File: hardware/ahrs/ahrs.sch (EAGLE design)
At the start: 32 parts, among them J1 2-PIN, U1 LSM9DS1, U2 STM32G4_UFQFPN48_T1, X1 NX2016SA24MHZ-EXS00A-CS11335, X2 SM08B-SRSS-TB

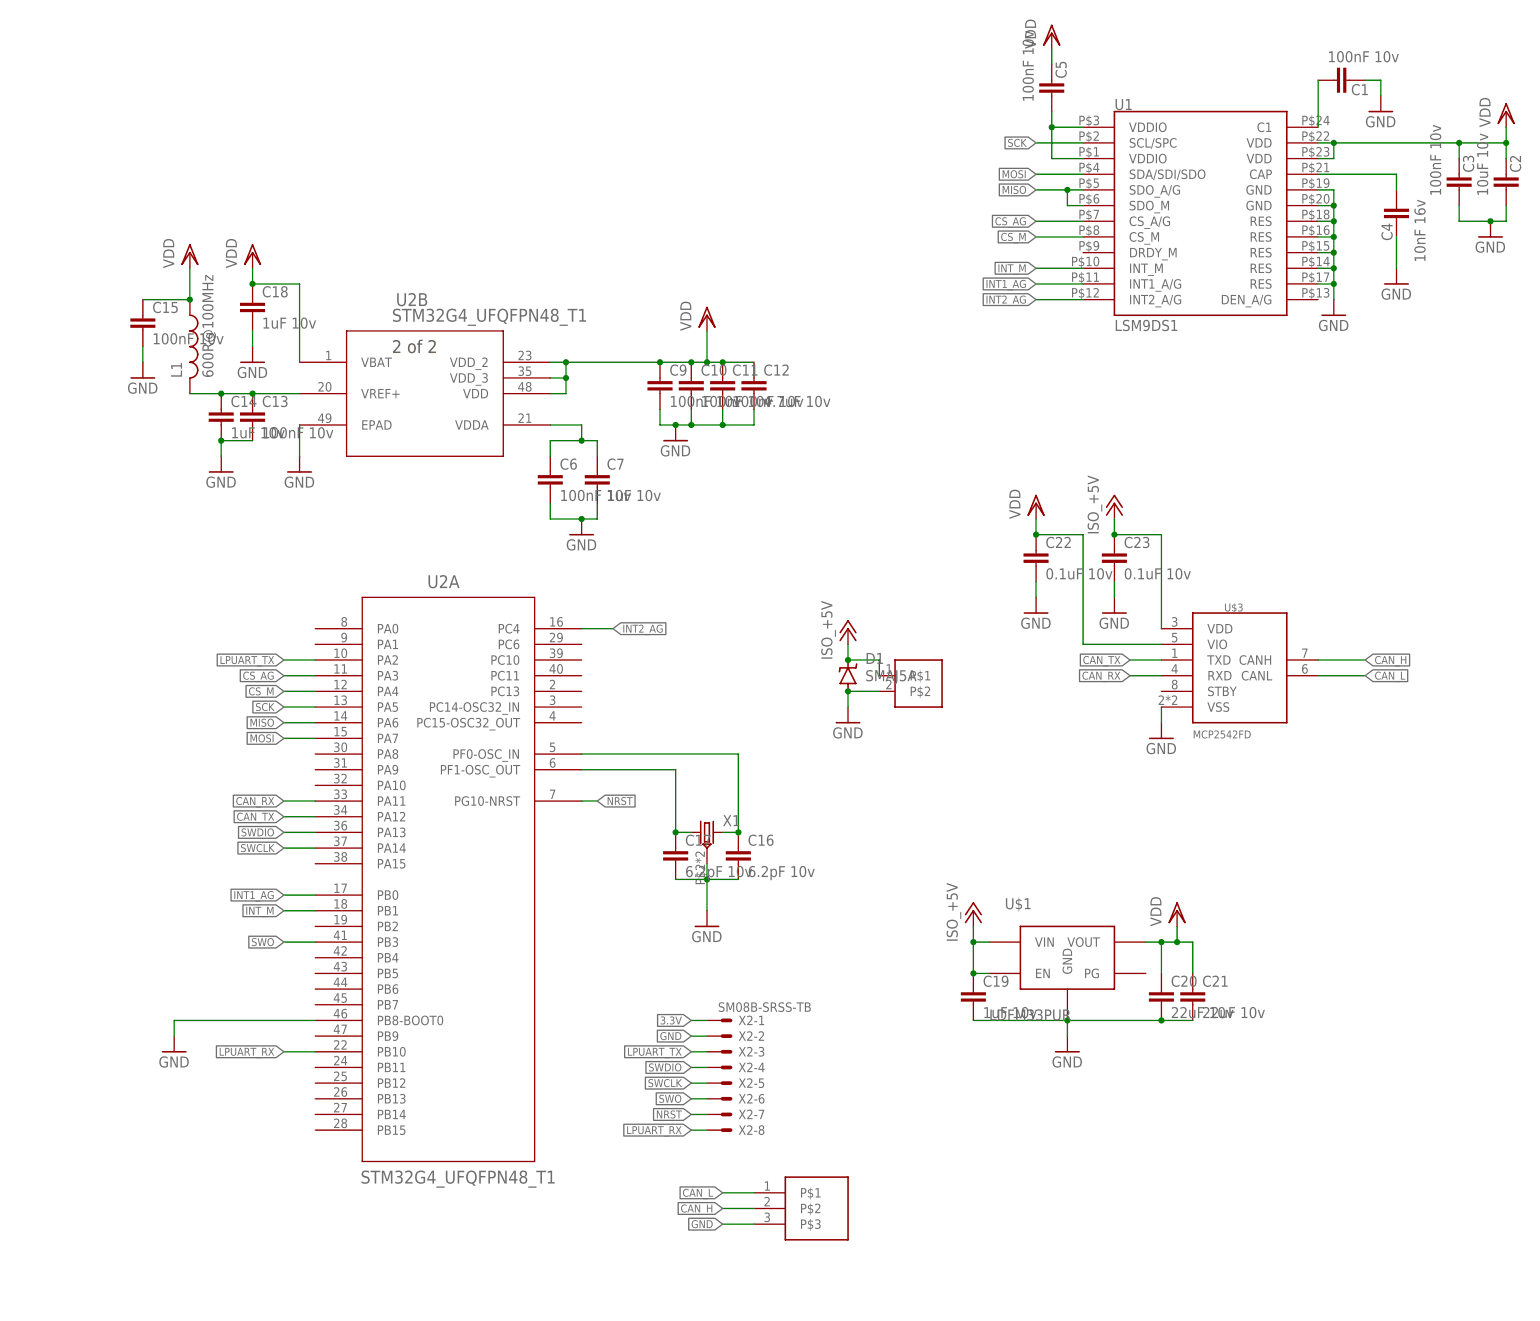
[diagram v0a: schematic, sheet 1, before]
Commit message: R1 of ahrs
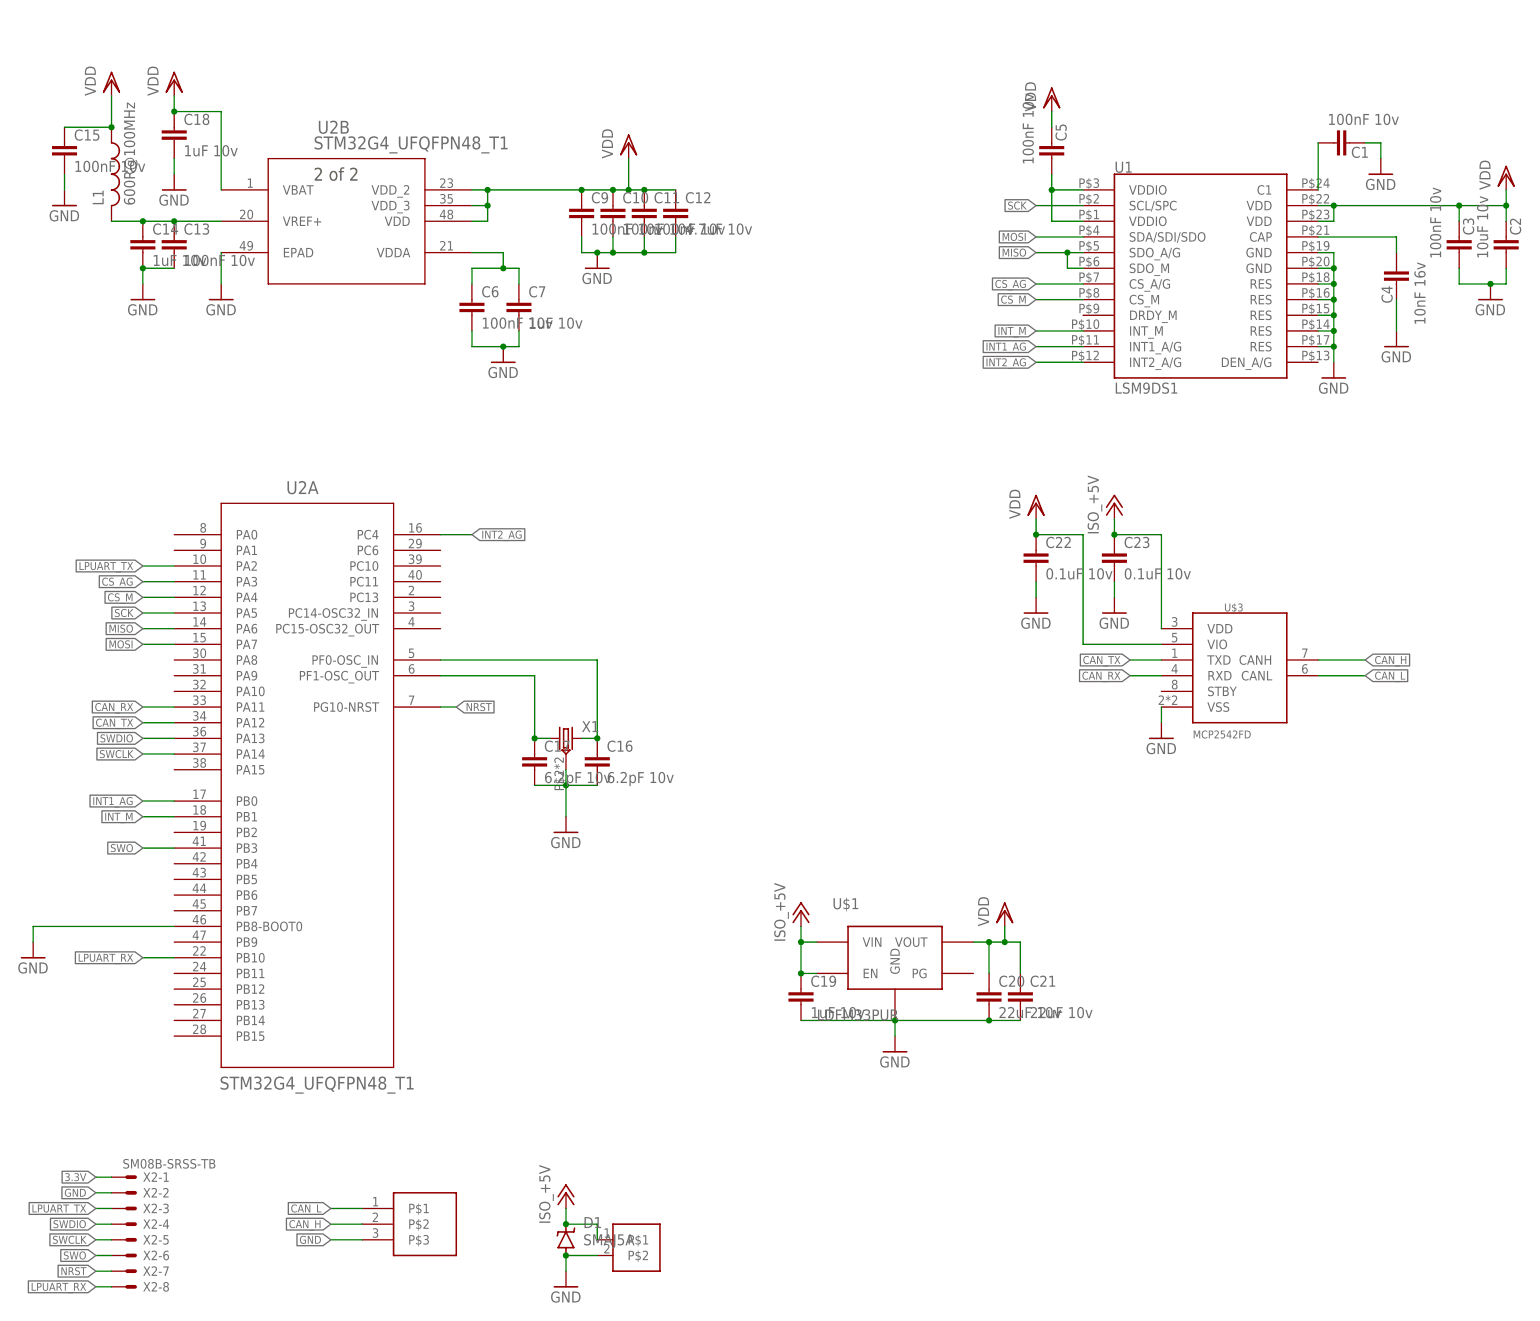
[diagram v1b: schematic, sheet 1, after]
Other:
- moved on the sheet: C1, C10, C11, C12, C13, C14, C15, C16, C17, C18, C19, C2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

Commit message: Prior to pulling from fusion
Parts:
- C1, C2, C3, C4, C5: device timlib:C_CERAMIC_0603 -> rcl:C-EUC0603
- X2: device con-jst2:SM08B-SRSS-TB -> timlib:SM08B-SRSS-TB
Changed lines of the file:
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@@
 <?xml version="1.0" encoding="utf-8"?>
 <!DOCTYPE eagle SYSTEM "eagle.dtd">
-<eagle version="9.5.2">
+<eagle version="9.6.1">
 <drawing>
 <settings>
@@
 <part name="FRAME1" library="frames" library_urn="urn:adsk.eagle:library:229" deviceset="FRAME_A_L" device=""/>
 <part name="U1" library="timlib" library_urn="urn:adsk.eagle:library:16152524" deviceset="LSM9DS1" device="" package3d_urn="urn:adsk.eagle:package:18130566/2"/>
-<part name="C1" library="timlib" library_urn="urn:adsk.eagle:library:16152524" deviceset="C_CERAMIC" device="_0603" package3d_urn="urn:adsk.eagle:package:23616/2" value="100nF 10v"/>
+<part name="C1" library="rcl" library_urn="urn:adsk.eagle:library:334" deviceset="C-EU" device="C0603" package3d_urn="urn:adsk.eagle:package:23616/2" value="100nF 10v"/>
 <part name="GND1" library="supply1" library_urn="urn:adsk.eagle:library:371" deviceset="GND" device=""/>
 <part name="VDD1" library="supply1" library_urn="urn:adsk.eagle:library:371" deviceset="VDD" device=""/>
 <part name="GND2" library="supply1" library_urn="urn:adsk.eagle:library:371" deviceset="GND" device=""/>
-<part name="C2" library="timlib" library_urn="urn:adsk.eagle:library:16152524" deviceset="C_CERAMIC" device="_0603" package3d_urn="urn:adsk.eagle:package:23616/2" value="10uF 10v"/>
-<part name="C3" library="timlib" library_urn="urn:adsk.eagle:library:16152524" deviceset="C_CERAMIC" device="_0603" package3d_urn="urn:adsk.eagle:package:23616/2" value="100nF 10v"/>
-<part name="C4" library="timlib" library_urn="urn:adsk.eagle:library:16152524" deviceset="C_CERAMIC" device="_0603" package3d_urn="urn:adsk.eagle:package:23616/2" value="10nF 16v"/>
+<part name="C2" library="rcl" library_urn="urn:adsk.eagle:library:334" deviceset="C-EU" device="C0603" package3d_urn="urn:adsk.eagle:package:23616/2" override_package3d_urn="urn:adsk.eagle:package:19477979/2" override_package_urn="urn:adsk.eagle:footprint:23123/1" value="10uF 10v"/>
+<part name="C3" library="rcl" library_urn="urn:adsk.eagle:library:334" deviceset="C-EU" device="C0603" package3d_urn="urn:adsk.eagle:package:23616/2" value="100nF 10v"/>
+<part name="C4" library="rcl" library_urn="urn:adsk.eagle:library:334" deviceset="C-EU" device="C0603" package3d_urn="urn:adsk.eagle:package:23616/2" value="10nF 16v"/>
 <part name="GND4" library="supply1" library_urn="urn:adsk.eagle:library:371" deviceset="GND" device=""/>
 <part name="VDD2" library="supply1" library_urn="urn:adsk.eagle:library:371" deviceset="VDD" device=""/>
-<part name="C5" library="timlib" library_urn="urn:adsk.eagle:library:16152524" deviceset="C_CERAMIC" device="_0603" package3d_urn="urn:adsk.eagle:package:23616/2" value="100nF 10v"/>
+<part name="C5" library="rcl" library_urn="urn:adsk.eagle:library:334" deviceset="C-EU" device="C0603" package3d_urn="urn:adsk.eagle:package:23616/2" value="100nF 10v"/>
 <part name="FRAME2" library="frames" library_urn="urn:adsk.eagle:library:229" deviceset="FRAME_A_L" device=""/>
-<part name="U2" library="timlib" library_urn="urn:adsk.eagle:library:16152524" deviceset="STM32G4_UFQFPN48_T1" device="" package3d_urn="urn:adsk.eagle:package:19324073/1"/>
+<part name="U2" library="timlib" library_urn="urn:adsk.eagle:library:16152524" deviceset="STM32G4_UFQFPN48_T1" device="" package3d_urn="urn:adsk.eagle:package:19324073/1" override_package3d_urn="urn:adsk.eagle:package:19324073/2" override_package_urn="urn:adsk.eagle:footprint:19324070/1"/>
 <part name="C6" library="rcl" library_urn="urn:adsk.eagle:library:334" deviceset="C-EU" device="C0603" package3d_urn="urn:adsk.eagle:package:23616/2" value="100nF 10v"/>
 <part name="C7" library="rcl" library_urn="urn:adsk.eagle:library:334" deviceset="C-EU" device="C0603" package3d_urn="urn:adsk.eagle:package:23616/2" value="1uF 10v"/>
@@
 <part name="U$5" library="timlib" library_urn="urn:adsk.eagle:library:16152524" deviceset="3-PIN" device="" package3d_urn="urn:adsk.eagle:package:16399489/2"/>
 <part name="GND15" library="supply1" library_urn="urn:adsk.eagle:library:371" deviceset="GND" device=""/>
-<part name="X2" library="con-jst2" library_urn="urn:adsk.eagle:library:19399826" deviceset="?M08B-SRSS-TB" device="S" package3d_urn="urn:adsk.eagle:package:19399895/1"/>
+<part name="X2" library="timlib" library_urn="urn:adsk.eagle:library:16152524" deviceset="?M08B-SRSS-TB" device="S" package3d_urn="urn:adsk.eagle:package:19399895/3"/>
 <part name="J1" library="timlib" library_urn="urn:adsk.eagle:library:16152524" deviceset="2-PIN" device="" package3d_urn="urn:adsk.eagle:package:16399492/4"/>
 <part name="GND16" library="supply1" library_urn="urn:adsk.eagle:library:371" deviceset="GND" device=""/>
@@
 will not be understood (or retained) with this version.
 </note>
+<note version="9.4" severity="warning">
+Since Version 9.4, EAGLE supports the overriding of 3D packages
+in schematics and board files. Those overridden 3d packages
+will not be understood (or retained) with this version.
+</note>

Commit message: Rerouting much better
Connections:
- net N$1 renamed VDDA
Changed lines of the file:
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@@
 <class number="0" name="default" width="0" drill="0">
+</class>
+<class number="1" name="power" width="0.3" drill="0">
 </class>
 </classes>
@@
 </busses>
 <nets>
-<net name="GND" class="0">
+<net name="GND" class="1">
 <segment>
 <pinref part="C1" gate="G$1" pin="1"/>
@@
 </segment>
 </net>
-<net name="3.3V" class="0">
+<net name="3.3V" class="1">
 <segment>
 <pinref part="U1" gate="G$1" pin="VDD@1"/>
@@
 </segment>
 </net>
-<net name="N$1" class="0">
+<net name="VDDA" class="1">
 <segment>
 <pinref part="C7" gate="G$1" pin="1"/>
@@
 </segment>
 </net>
-<net name="VREF" class="0">
+<net name="VREF" class="1">
 <segment>
 <pinref part="C14" gate="G$1" pin="1"/>
@@
 </segment>
 </net>
-<net name="5V" class="0">
+<net name="5V" class="1">
 <segment>
 <pinref part="U$1" gate="G$1" pin="VIN"/>
